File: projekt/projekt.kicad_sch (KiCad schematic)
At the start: 22 parts, among them J1 S8421-45R, SW1 SW_Push, U1 NE555P

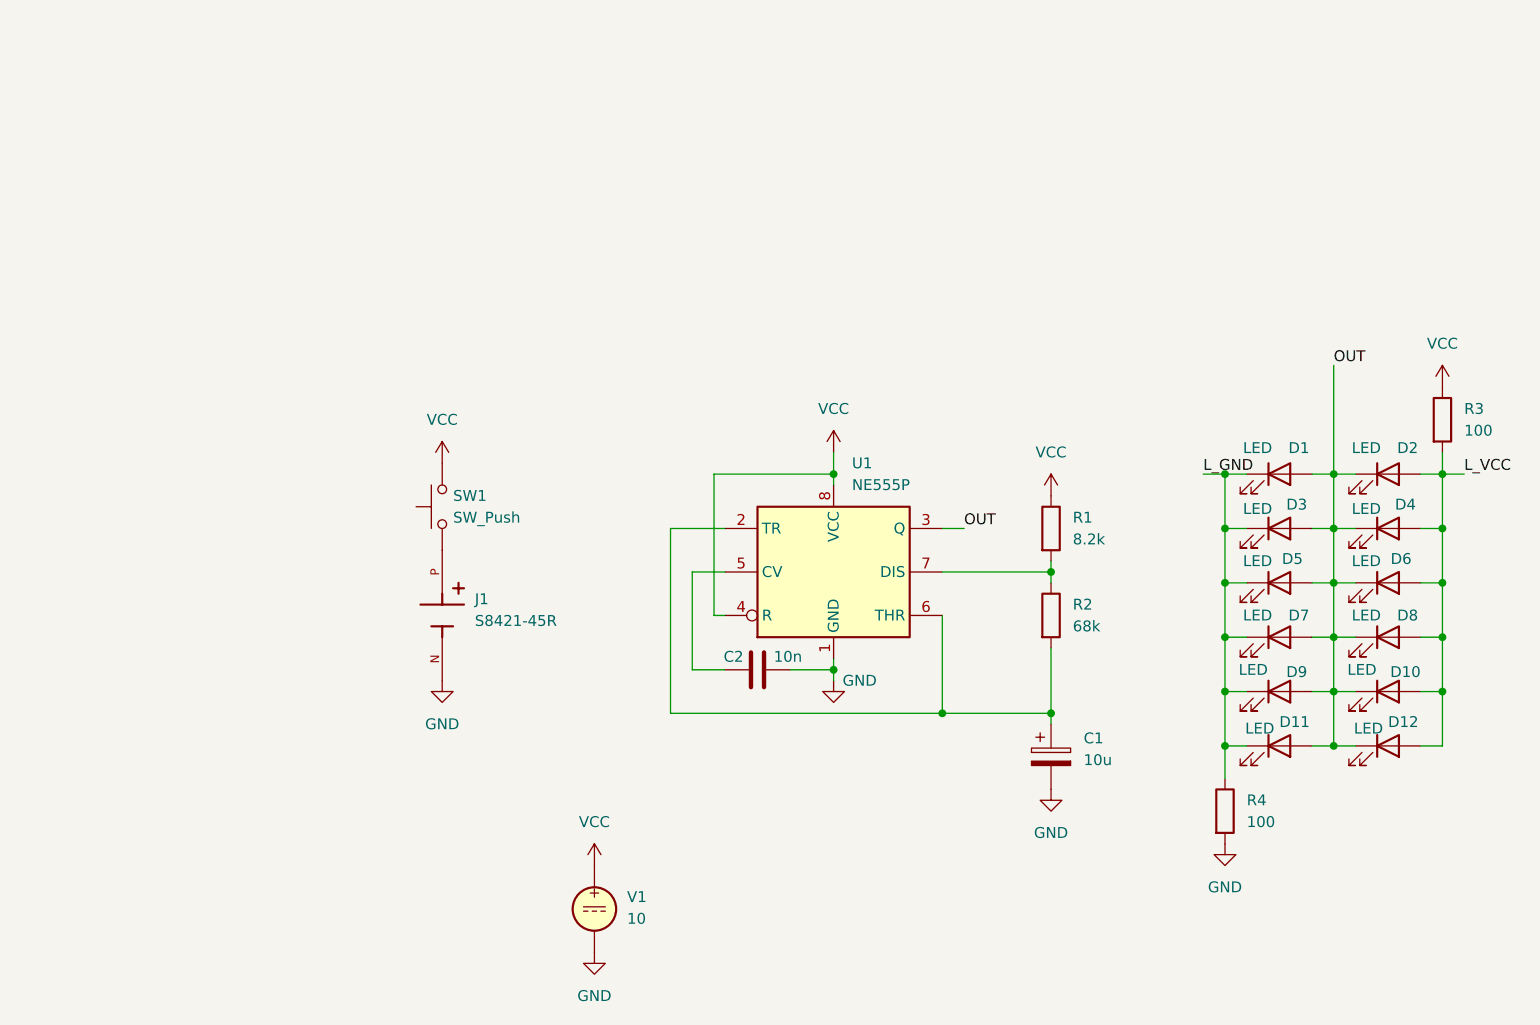
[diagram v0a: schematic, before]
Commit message: zdjęcia i wgl
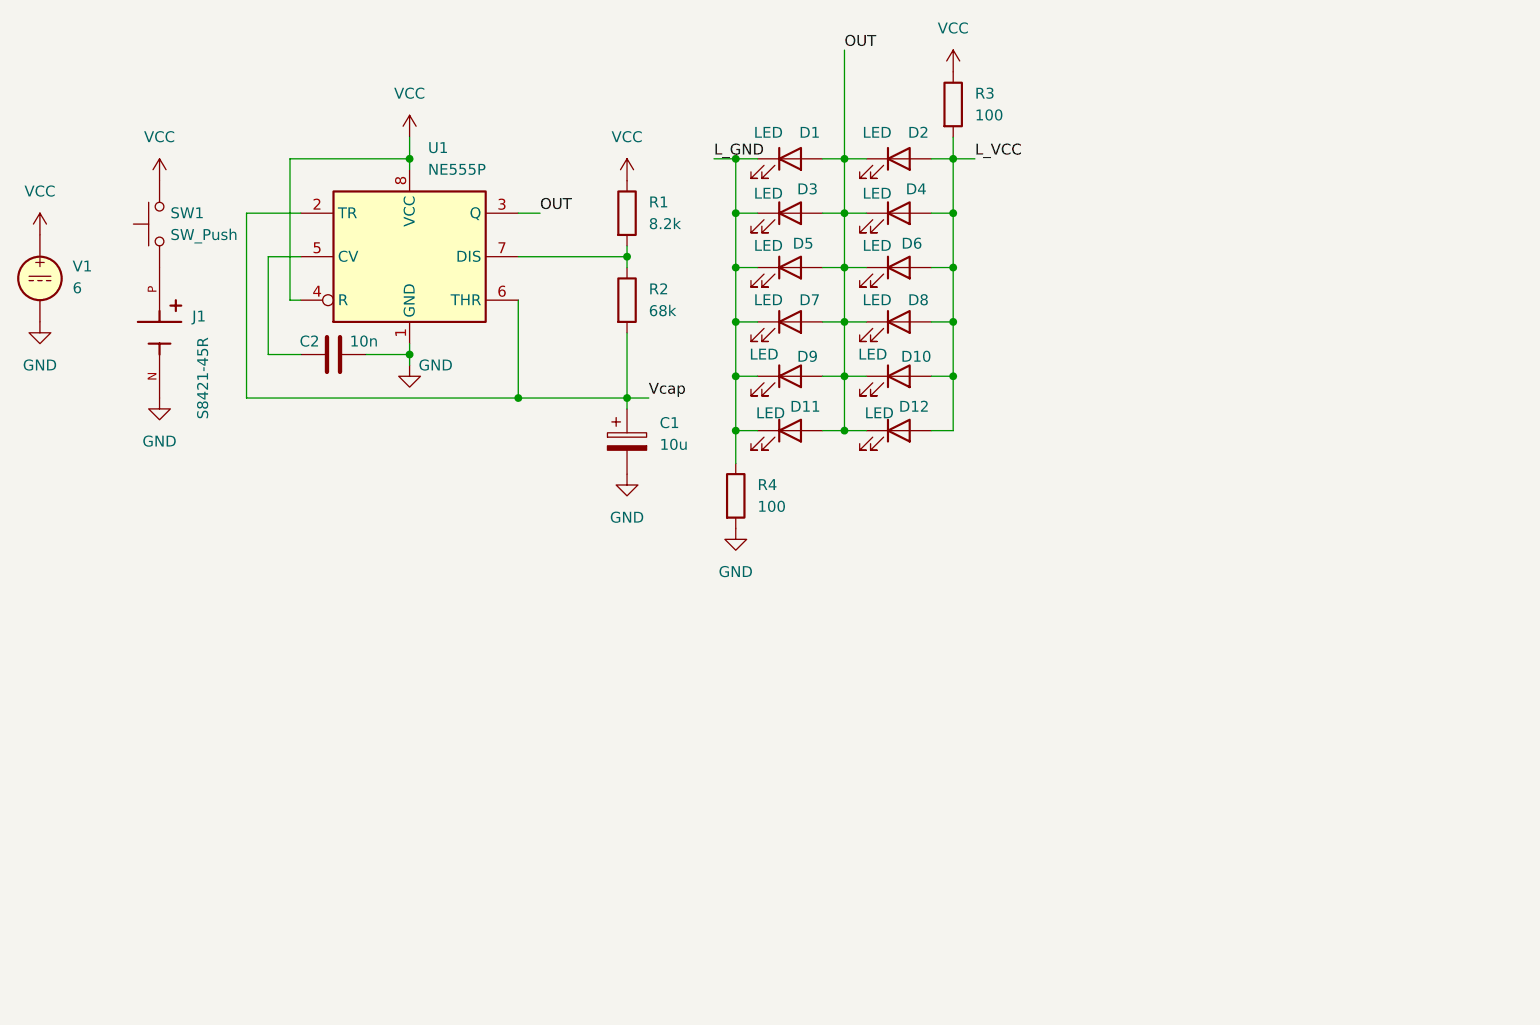
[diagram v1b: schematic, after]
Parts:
- V1: value 10 -> 6
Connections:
- net Vcap: now reaches C1.1, R2.2, U1.2 (TR), U1.6 (THR)
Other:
- moved on the sheet: C1, C2, D1, D10, D11, D12, D2, D3, D4, D5, D6, D7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
